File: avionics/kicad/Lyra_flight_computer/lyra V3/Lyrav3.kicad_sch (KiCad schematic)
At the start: 84 parts, among them J2 Screw_Terminal_01x06, J3 Conn_01x02, J4 Conn_01x02, J5 Conn_01x03, J6 Conn_01x06, J7 USB_B_Micro, J8 Conn_01x04, J9 Screw_Terminal_01x06, Q1 AO3401A, Q2 AO3400A, Q3 AO3400A, Q4 AO3400A, Q5 AO3400A, U1 AZ1117-3.3, U2 BMI088, U3 MPL3115A2, U4 ADXL375BCCZ-RL7, U5 LIS3MDL, U6 ADS1015IDGS, U7 W25Q64JVXGIQ, U8 RP2040, X1 S3D12.288000B20F30T

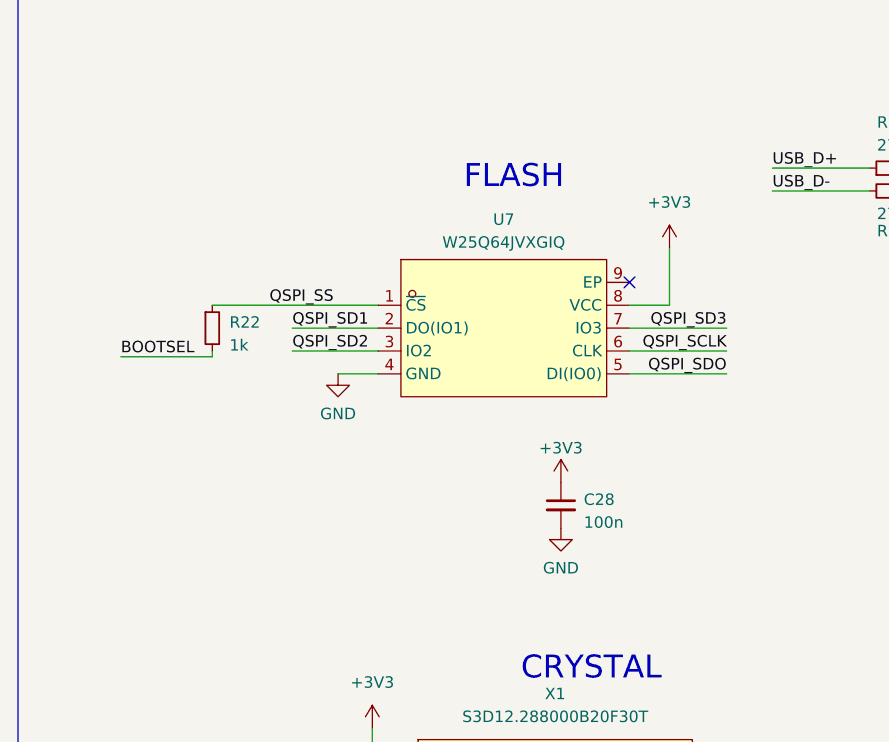
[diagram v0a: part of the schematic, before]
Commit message: real pretrip
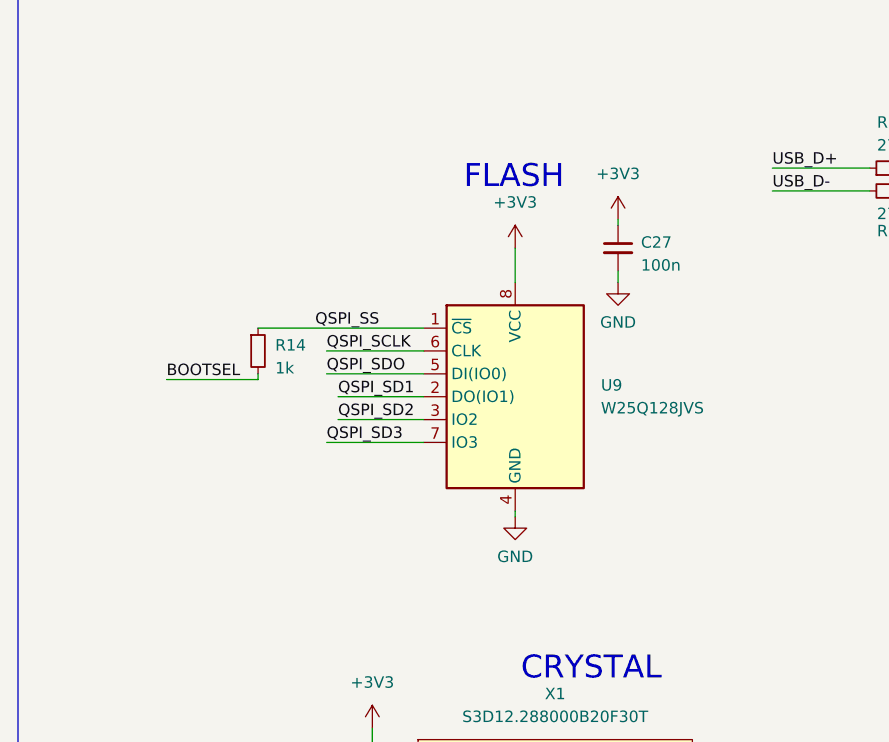
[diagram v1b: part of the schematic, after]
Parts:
- removed C28: 100n, Capacitor_SMD:C_0603_1608Metric, symbol Device:C_Small
- removed R22: 1k, Resistor_SMD:R_0603_1608Metric, symbol Device:R_Small
- removed U7: W25Q64JVXGIQ, Package_SO:SOIC-8_5.23x5.23mm_P1.27mm, symbol easyeda2kicad:W25Q64JVXGIQ
- added C27: 100n, Capacitor_SMD:C_0603_1608Metric, symbol Device:C_Small
- added R14: 1k, Resistor_SMD:R_0603_1608Metric, symbol Device:R_Small
- added U9: W25Q128JVS, Package_SO:SOIC-8_5.23x5.23mm_P1.27mm, symbol Memory_Flash:W25Q128JVS
- J5: LCSC Part C160403 -> (none)
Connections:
- net +3V3: now also C27.1, U9.8 (VCC)
- net BOOTSEL: now also R14.2
- net GND: now also C27.2, U9.4 (GND)
- net QSPI_SCLK: now also U9.6 (CLK)
- net QSPI_SD1: now also U9.2 (DO(IO1))
- net QSPI_SD2: now also U9.3 (IO2)
- net QSPI_SD3: now also U9.7 (IO3)
- net QSPI_SDO: now also U9.5 (DI(IO0))
- net QSPI_SS: now also R14.1, U9.1 (~{CS})
- no-connect marks 30 -> 29
